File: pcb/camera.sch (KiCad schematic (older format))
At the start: 17 parts, among them IC3 EL817S, IC4 EL817S, IC7 EL817S, IC8 EL817S, J1 SJ-2523-SMT-TR

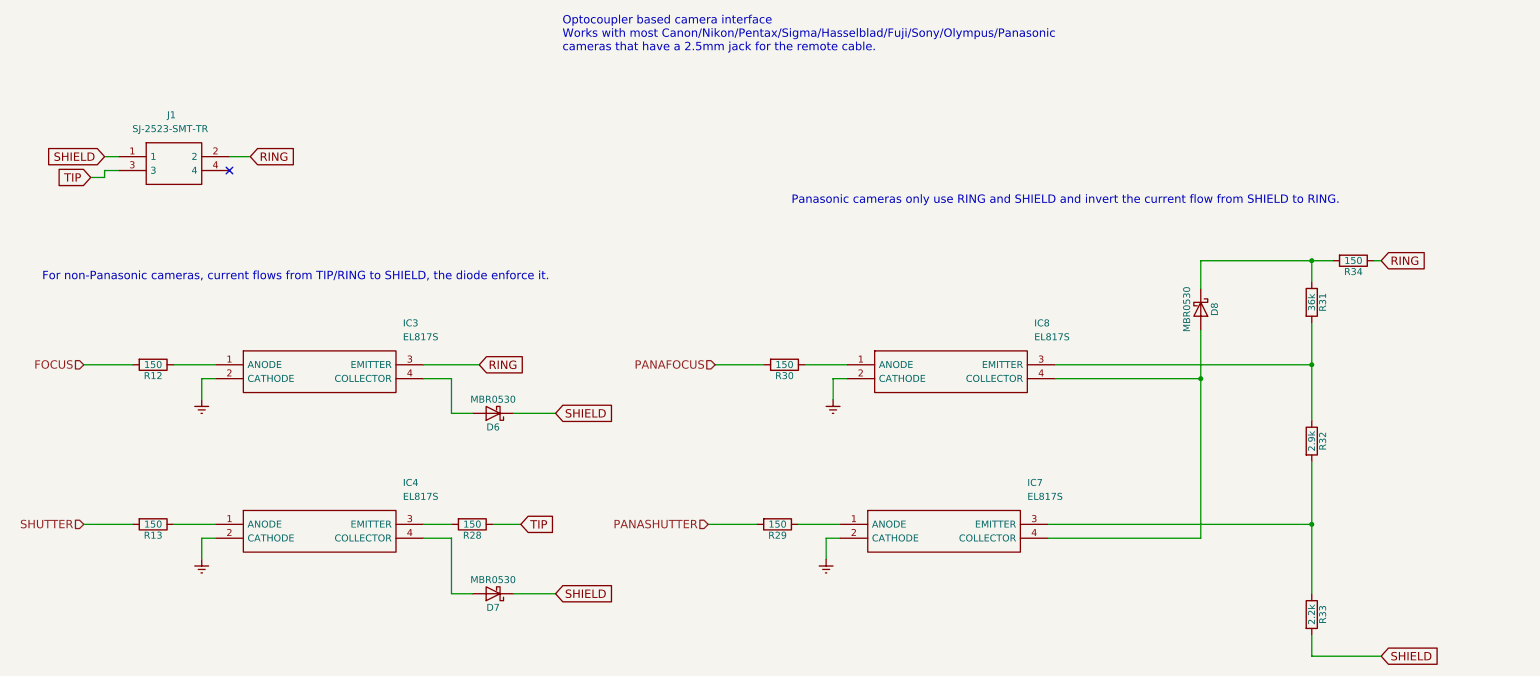
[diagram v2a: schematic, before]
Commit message: v0.1 Prototype files sent to PCBWay
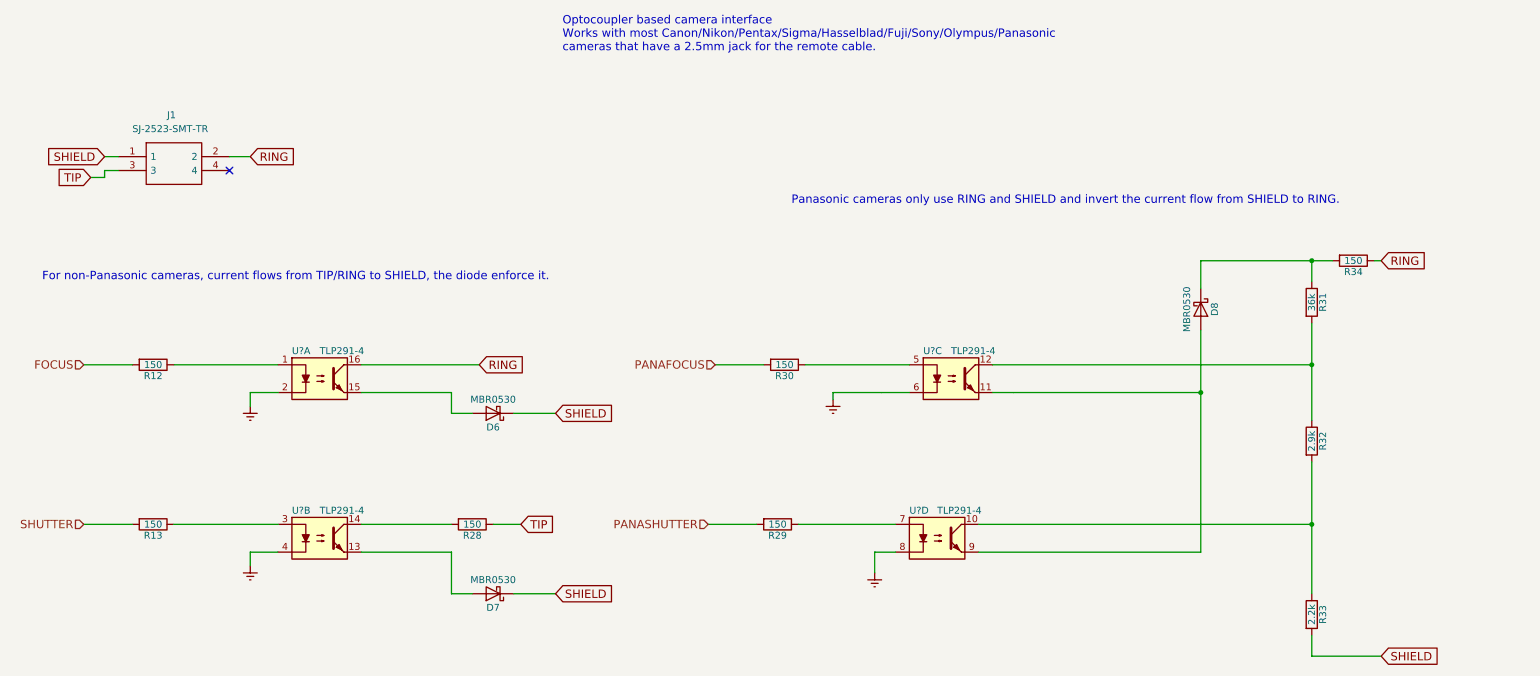
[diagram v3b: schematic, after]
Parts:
- removed IC3, IC4, IC7, IC8: EL817S, EL817S:EL817S, symbol EL817S
- added U? (x4): TLP291-4, Housings_DIP:DIP-16_W7.62mm_SMD, symbol TLP291-4
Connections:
- net Earth: now also U?.2, U?.4, U?.6, U?.8
- net RING: now also U?.16
- net at R12.1: now also U?.1
- net at D6.2 (A): now also U?.15
- net at R13.1: now also U?.3
- net at R28.2: now also U?.14
- net at D7.2 (A): now also U?.13
- net at R30.1: now also U?.5
- net at R31.2, R32.1: now also U?.12
- net at D8.2 (A): now also U?.11, U?.9
- net at R29.1: now also U?.7
- net at R32.2, R33.1: now also U?.10
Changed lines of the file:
@@
 LIBS:xilinx
 LIBS:zetex
+LIBS:SparkFun
+LIBS:ab2_7segment
+LIBS:ab2_audio
+LIBS:ab2_buffer
+LIBS:ab2_capacitor
+LIBS:ab2_connectivity
+LIBS:ab2_dac
+LIBS:ab2_diode
+LIBS:ab2_fuse
+LIBS:ab2_gpio_expansion
+LIBS:ab2_header
+LIBS:ab2_idc
+LIBS:ab2_inductor
+LIBS:ab2_input_devices
+LIBS:ab2_jumper
+LIBS:ab2_lcd
+LIBS:ab2_led
+LIBS:ab2_memory
+LIBS:ab2_opamp
+LIBS:ab2_pinouts
+LIBS:ab2_pot
+LIBS:ab2_power
+LIBS:ab2_regulator
+LIBS:ab2_relay
+LIBS:ab2_resistor
+LIBS:ab2_sensor
+LIBS:ab2_stepper
+LIBS:ab2_supply
+LIBS:ab2_terminal_block
+LIBS:ab2_test
+LIBS:ab2_transistor
+LIBS:ab2_uC
+LIBS:ab2_usb
+LIBS:ab2_xtal
 LIBS:EL817S
 LIBS:IRA-S210ST01
@@
 TIP
 Wire Wire Line
-	2000 3800 2300 3800
+	2000 3800 2750 3800
 Text GLabel 4200 3800 2    60   Input ~ 0
 RING
 Wire Wire Line
-	3800 3800 4200 3800
+	3350 3800 4200 3800
 Text GLabel 4750 4150 2    60   Input ~ 0
 SHIELD
@@
 L Earth #PWR014
 U 1 1 5A80CEBC
-P 2200 4050
-F 0 "#PWR014" H 2200 3800 50  0001 C CNN
-F 1 "Earth" H 2200 3900 50  0001 C CNN
-F 2 "" H 2200 4050 50  0001 C CNN
-F 3 "" H 2200 4050 50  0001 C CNN
-	1    2200 4050
-	1    0    0    -1
-$EndComp
-Wire Wire Line
-	2200 4050 2200 3900
-Wire Wire Line
-	2200 3900 2300 3900
+P 2550 4100
+F 0 "#PWR014" H 2550 3850 50  0001 C CNN
+F 1 "Earth" H 2550 3950 50  0001 C CNN
+F 2 "" H 2550 4100 50  0001 C CNN
+F 3 "" H 2550 4100 50  0001 C CNN
+	1    2550 4100
+	1    0    0    -1
+$EndComp
 $Comp
 L R R12
@@
 SHUTTER
 Wire Wire Line
-	2000 4950 2300 4950
+	2000 4950 2750 4950
 Text GLabel 4500 4950 2    60   Input ~ 0
 TIP
@@
 SHIELD
 $Comp
-L EL817S IC4
-U 1 1 5A80D1A3
-P 2300 4950
-F 0 "IC4" H 3650 5250 50  0000 L CNN
-F 1 "EL817S" H 3650 5150 50  0000 L CNN
-F 2 "EL817S:EL817S" H 3650 5050 50  0001 L CNN
-F 3 "http://www.mouser.com/ds/2/143/201407061833256242-365628.pdf" H 3650 4950 50  0001 L CNN
-F 4 "Transistor Output Optocouplers Photo-Coupler" H 3650 4850 50  0001 L CNN "Description"
-F 5 "Everlight" H 3650 4750 50  0001 L CNN "Manufacturer_Name"
-F 6 "EL817S" H 3650 4650 50  0001 L CNN "Manufacturer_Part_Number"
-F 7 "RS" H 3650 4550 50  0001 L CNN "Supplier_Name"
-F 8 "" H 3650 4450 50  0001 L CNN "RS Part Number"
-F 9 "" H 3650 4350 50  0001 L CNN "Height"
-	1    2300 4950
-	1    0    0    -1
-$EndComp
-$Comp
 L Earth #PWR015
 U 1 1 5A80D1A9
-P 2200 5200
-F 0 "#PWR015" H 2200 4950 50  0001 C CNN
-F 1 "Earth" H 2200 5050 50  0001 C CNN
-F 2 "" H 2200 5200 50  0001 C CNN
-F 3 "" H 2200 5200 50  0001 C CNN
-	1    2200 5200
-	1    0    0    -1
-$EndComp
-Wire Wire Line
-	2200 5200 2200 5050
-Wire Wire Line
-	2200 5050 2300 5050
+P 2550 5250
+F 0 "#PWR015" H 2550 5000 50  0001 C CNN
+F 1 "Earth" H 2550 5100 50  0001 C CNN
+F 2 "" H 2550 5250 50  0001 C CNN
+F 3 "" H 2550 5250 50  0001 C CNN
+	1    2550 5250
+	1    0    0    -1
+$EndComp
 $Comp
 L R R13
@@
 PANAFOCUS
 Wire Wire Line
-	6550 3800 6850 3800
+	6550 3800 7300 3800
 Text GLabel 10700 3050 2    60   Input ~ 0
 RING
 Text GLabel 10700 5900 2    60   Input ~ 0
 SHIELD
-$Comp
-L EL817S IC8
-U 1 1 5A83904A
-P 6850 3800
-F 0 "IC8" H 8200 4100 50  0000 L CNN
-F 1 "EL817S" H 8200 4000 50  0000 L CNN
-F 2 "EL817S:EL817S" H 8200 3900 50  0001 L CNN
-F 3 "http://www.mouser.com/ds/2/143/201407061833256242-365628.pdf" H 8200 3800 50  0001 L CNN
-F 4 "Transistor Output Optocouplers Photo-Coupler" H 8200 3700 50  0001 L CNN "Description"
-F 5 "Everlight" H 8200 3600 50  0001 L CNN "Manufacturer_Name"
-F 6 "EL817S" H 8200 3500 50  0001 L CNN "Manufacturer_Part_Number"
-F 7 "RS" H 8200 3400 50  0001 L CNN "Supplier_Name"
-F 8 "" H 8200 3300 50  0001 L CNN "RS Part Number"
-F 9 "" H 8200 3200 50  0001 L CNN "Height"
-	1    6850 3800
-	1    0    0    -1
-$EndComp
 $Comp
 L Earth #PWR016
@@
 $EndComp
 Wire Wire Line
-	6750 4050 6750 3900
-Wire Wire Line
-	6750 3900 6850 3900
+	6750 4050 6750 4000
+Wire Wire Line
+	6750 4000 7100 4000
 $Comp
 L R R30
@@
 PANASHUTTER
 Wire Wire Line
-	6500 4950 6800 4950
-$Comp
-L EL817S IC7
-U 1 1 5A839193
-P 6800 4950
-F 0 "IC7" H 8150 5250 50  0000 L CNN
-F 1 "EL817S" H 8150 5150 50  0000 L CNN
-F 2 "EL817S:EL817S" H 8150 5050 50  0001 L CNN
-F 3 "http://www.mouser.com/ds/2/143/201407061833256242-365628.pdf" H 8150 4950 50  0001 L CNN
-F 4 "Transistor Output Optocouplers Photo-Coupler" H 8150 4850 50  0001 L CNN "Description"
-F 5 "Everlight" H 8150 4750 50  0001 L CNN "Manufacturer_Name"
-F 6 "EL817S" H 8150 4650 50  0001 L CNN "Manufacturer_Part_Number"
-F 7 "RS" H 8150 4550 50  0001 L CNN "Supplier_Name"
-F 8 "" H 8150 4450 50  0001 L CNN "RS Part Number"
-F 9 "" H 8150 4350 50  0001 L CNN "Height"
-	1    6800 4950
-	1    0    0    -1
-$EndComp
+	6500 4950 7200 4950
 $Comp
 L Earth #PWR017
 U 1 1 5A839199
-P 6700 5200
-F 0 "#PWR017" H 6700 4950 50  0001 C CNN
-F 1 "Earth" H 6700 5050 50  0001 C CNN
-F 2 "" H 6700 5200 50  0001 C CNN
-F 3 "" H 6700 5200 50  0001 C CNN
-	1    6700 5200
-	1    0    0    -1
-$EndComp
-Wire Wire Line
-	6700 5200 6700 5050
-Wire Wire Line
-	6700 5050 6800 5050
+P 7050 5300
+F 0 "#PWR017" H 7050 5050 50  0001 C CNN
+F 1 "Earth" H 7050 5150 50  0001 C CNN
+F 2 "" H 7050 5300 50  0001 C CNN
+F 3 "" H 7050 5300 50  0001 C CNN
+	1    7050 5300
+	1    0    0    -1
+$EndComp
+Wire Wire Line
+	7050 5300 7050 5150
+Wire Wire Line
+	7050 5150 7200 5150
 $Comp
 L R R29
@@
 $EndComp
 Wire Wire Line
-	10200 4500 10200 5450
-Wire Wire Line
-	10200 3500 10200 4200
+	10200 4500 10200 4950
+Wire Wire Line
+	10200 4950 10200 5450
+Wire Wire Line
+	10200 3500 10200 3800
+Wire Wire Line
+	10200 3800 10200 4200
 Wire Wire Line
 	10200 5750 10200 5900
@@
 	10200 5900 10700 5900
 Wire Wire Line
-	9400 3050 10350 3050
+	9400 3050 10200 3050
+Wire Wire Line
+	10200 3050 10350 3050
 Wire Wire Line
 	10200 3050 10200 3200
 Wire Wire Line
-	10200 3800 8350 3800
+	7900 3800 10200 3800
 Connection ~ 10200 3800
 Wire Wire Line
-	8350 3900 9400 3900
-Wire Wire Line
-	9400 3550 9400 5050
-Wire Wire Line
-	10200 4950 8300 4950
+	8050 4000 9400 4000
+Wire Wire Line
+	9400 3550 9400 4000
+Wire Wire Line
+	9400 4000 9400 5150
+Wire Wire Line
+	7800 4950 10200 4950
 Connection ~ 10200 4950
-Wire Wire Line
-	9400 5050 8300 5050
 $Comp
 L MBR0530 D8
@@
 $EndComp
 Wire Wire Line
-	3800 3900 4000 3900
-Wire Wire Line
-	4000 3900 4000 4150
-Wire Wire Line
 	4000 4150 4150 4150
 Wire Wire Line
@@
 $EndComp
 Wire Wire Line
-	3800 5050 4000 5050
-Wire Wire Line
-	4000 5050 4000 5450
-Wire Wire Line
 	4000 5450 4150 5450
 Wire Wire Line
@@
 $EndComp
 Wire Wire Line
-	3800 4950 4000 4950
+	3350 4950 4000 4950
 Wire Wire Line
 	4300 4950 4500 4950
-Connection ~ 9400 3900
+Connection ~ 9400 4000
 Wire Wire Line
 	9400 3250 9400 3050
@@
 NoConn ~ 2400 2400
 $Comp
-L EL817S IC3
-U 1 1 5A80CC0F
-P 2300 3800
-F 0 "IC3" H 3650 4100 50  0000 L CNN
-F 1 "EL817S" H 3650 4000 50  0000 L CNN
-F 2 "EL817S:EL817S" H 3650 3900 50  0001 L CNN
-F 3 "http://www.mouser.com/ds/2/143/201407061833256242-365628.pdf" H 3650 3800 50  0001 L CNN
-F 4 "Transistor Output Optocouplers Photo-Coupler" H 3650 3700 50  0001 L CNN "Description"
-F 5 "Everlight" H 3650 3600 50  0001 L CNN "Manufacturer_Name"
-F 6 "EL817S" H 3650 3500 50  0001 L CNN "Manufacturer_Part_Number"
-F 7 "RS" H 3650 3400 50  0001 L CNN "Supplier_Name"
-F 8 "" H 3650 3300 50  0001 L CNN "RS Part Number"
-F 9 "" H 3650 3200 50  0001 L CNN "Height"
-	1    2300 3800
-	1    0    0    -1
-$EndComp
+L TLP291-4 U?
+U 1 1 5A90E6D4
+P 3050 3900
+F 0 "U?" H 2850 4100 50  0000 L CNN
+F 1 "TLP291-4" H 3050 4100 50  0000 L CNN
+F 2 "Housings_DIP:DIP-16_W7.62mm_SMD" H 2850 3700 50  0001 L CIN
+F 3 "" H 3050 3900 50  0001 L CNN
+	1    3050 3900
+	1    0    0    -1
+$EndComp
+$Comp
+L TLP291-4 U?
+U 2 1 5A90E755
+P 3050 5050
+F 0 "U?" H 2850 5250 50  0000 L CNN
+F 1 "TLP291-4" H 3050 5250 50  0000 L CNN
+F 2 "Housings_DIP:DIP-16_W7.62mm_SMD" H 2850 4850 50  0001 L CIN
+F 3 "" H 3050 5050 50  0001 L CNN
+	2    3050 5050
+	1    0    0    -1
+$EndComp
+$Comp
+L TLP291-4 U?
+U 3 1 5A90E7DE
+P 7600 3900
+F 0 "U?" H 7400 4100 50  0000 L CNN
+F 1 "TLP291-4" H 7600 4100 50  0000 L CNN
+F 2 "Housings_DIP:DIP-16_W7.62mm_SMD" H 7400 3700 50  0001 L CIN
+F 3 "" H 7600 3900 50  0001 L CNN
+	3    7600 3900
+	1    0    0    -1
+$EndComp
+$Comp
+L TLP291-4 U?
+U 4 1 5A90E8A6
+P 7500 5050
+F 0 "U?" H 7300 5250 50  0000 L CNN
+F 1 "TLP291-4" H 7500 5250 50  0000 L CNN
+F 2 "Housings_DIP:DIP-16_W7.62mm_SMD" H 7300 4850 50  0001 L CIN
+F 3 "" H 7500 5050 50  0001 L CNN
+	4    7500 5050
+	1    0    0    -1
+$EndComp
+Wire Wire Line
+	2550 4100 2550 4000
+Wire Wire Line
+	2550 4000 2750 4000
+Wire Wire Line
+	3350 4000 4000 4000
+Wire Wire Line
+	4000 4000 4000 4150
+Wire Wire Line
+	2550 5250 2550 5150
+Wire Wire Line
+	2550 5150 2750 5150
+Wire Wire Line
+	3350 5150 4000 5150
+Wire Wire Line
+	4000 5150 4000 5450
+Wire Wire Line
+	7100 4000 7100 4000
+Wire Wire Line
+	7100 4000 7300 4000
+Wire Wire Line
+	7900 4000 8050 4000
+Wire Wire Line
+	8050 4000 8050 4000
+Wire Wire Line
+	9400 5150 7800 5150
 $EndSCHEMATC
